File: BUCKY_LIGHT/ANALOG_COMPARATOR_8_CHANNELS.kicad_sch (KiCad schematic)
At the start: 12 parts, among them IC15 LM319N_NOPB, IC16 LM319N_NOPB, IC17 LM319N_NOPB, IC18 LM319N_NOPB

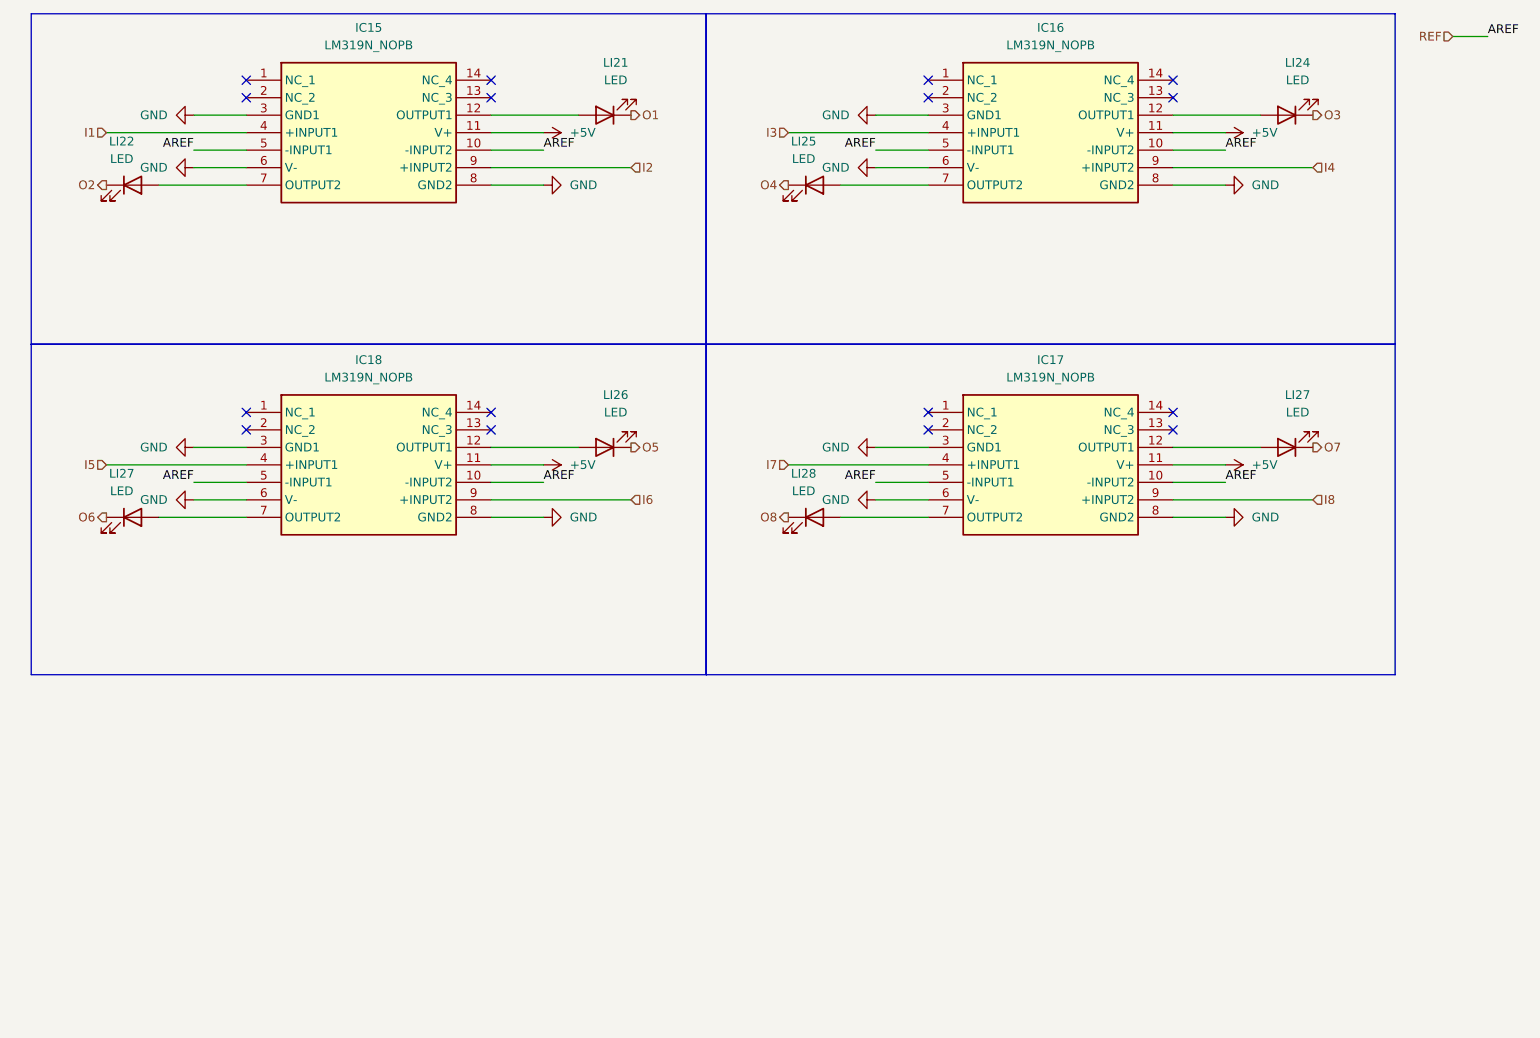
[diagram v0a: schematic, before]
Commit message: finish up robot (i think)
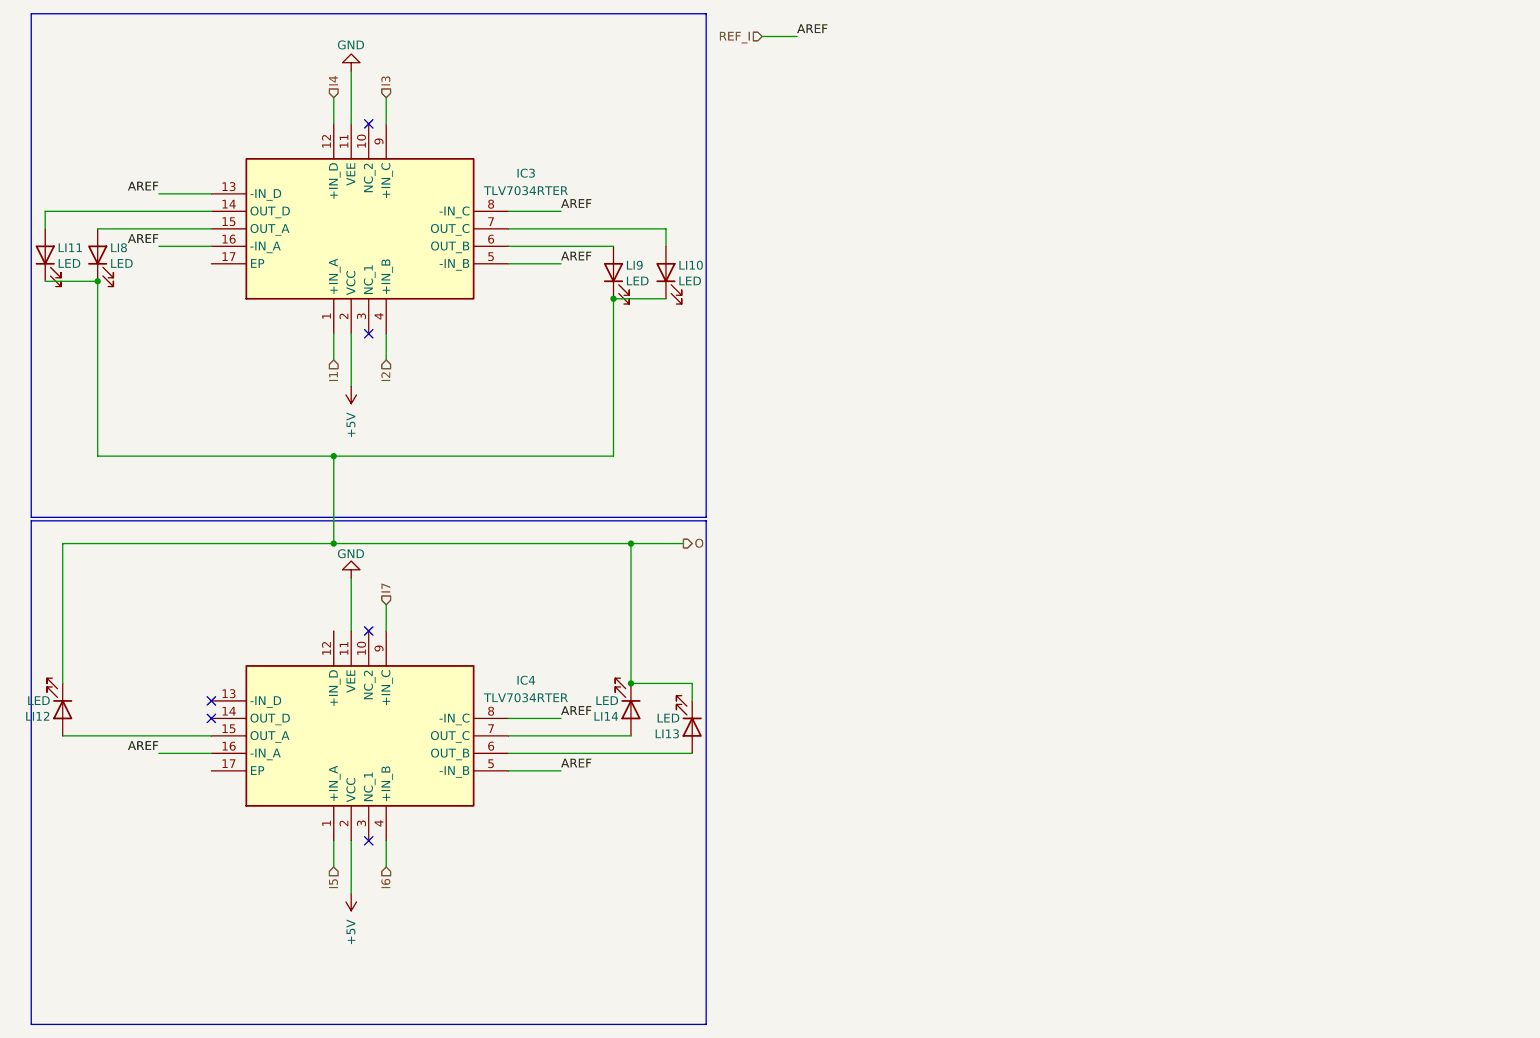
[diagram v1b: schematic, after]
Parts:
- removed IC15, IC16, IC17, IC18: LM319N_NOPB, DIP794W56P254L1905H533Q14N, symbol ANALOG_COMP:LM319N_NOPB
- removed LI21, LI22, LI24, LI25, LI26, LI27 (x2), LI28: LED, symbol Device:LED
- added IC3, IC4: TLV7034RTER, BUCKY_LIGHT:ANALOG_COMP, symbol ANALOG_COMP:TLV7034RTER
- added LI10, LI11, LI12, LI13, LI14, LI8, LI9: LED, LED_SMD:LED_0603_1608Metric, symbol Device:LED
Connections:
- net +5V: now also IC3.2 (VCC), IC4.2 (VCC)
- net GND: now also IC3.11 (VEE), IC4.11 (VEE)
- net I1: now also IC3.1 (+IN_A)
- net I2: now also IC3.4 (+IN_B)
- net I3: now also IC3.9 (+IN_C)
- net I4: now also IC3.12 (+IN_D)
- net I5: now also IC4.1 (+IN_A)
- net I6: now also IC4.4 (+IN_B)
- net I7: now also IC4.9 (+IN_C)
- new net: IC4.15 (OUT_A), LI12.2 (A)
- new net: IC3.14 (OUT_D), LI11.2 (A)
- new net: IC3.15 (OUT_A), LI8.2 (A)
- new net: IC3.6 (OUT_B), LI9.2 (A)
- new net: IC3.7 (OUT_C), LI10.2 (A)
- new net: IC4.6 (OUT_B), LI13.2 (A)
- new net: IC4.7 (OUT_C), LI14.2 (A)
- new net O: LI10.1 (K), LI11.1 (K), LI12.1 (K), LI13.1 (K), LI14.1 (K), LI8.1 (K), LI9.1 (K)
- new net REF_I: IC3.13 (-IN_D), IC3.16 (-IN_A), IC3.5 (-IN_B), IC3.8 (-IN_C), IC4.16 (-IN_A), IC4.5 (-IN_B), IC4.8 (-IN_C)
- no-connect marks 16 -> 6
